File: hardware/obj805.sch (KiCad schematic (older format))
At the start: 37 parts, among them J0 Conn_with_rapi, U1 l293d

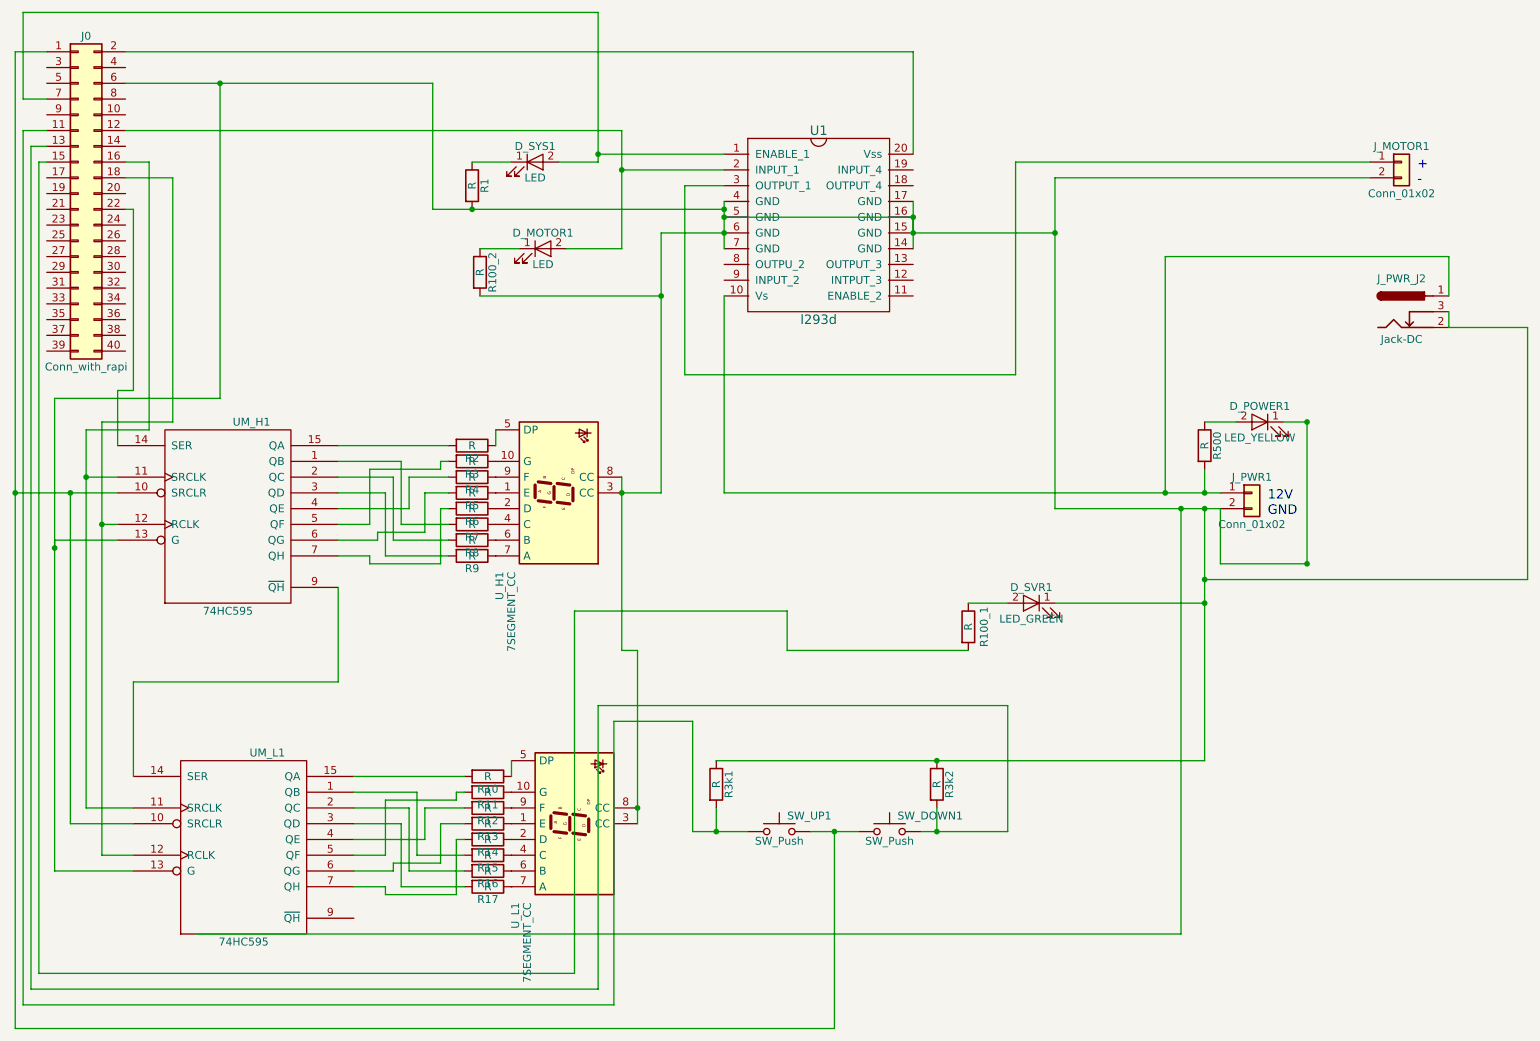
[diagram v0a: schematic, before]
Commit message: update
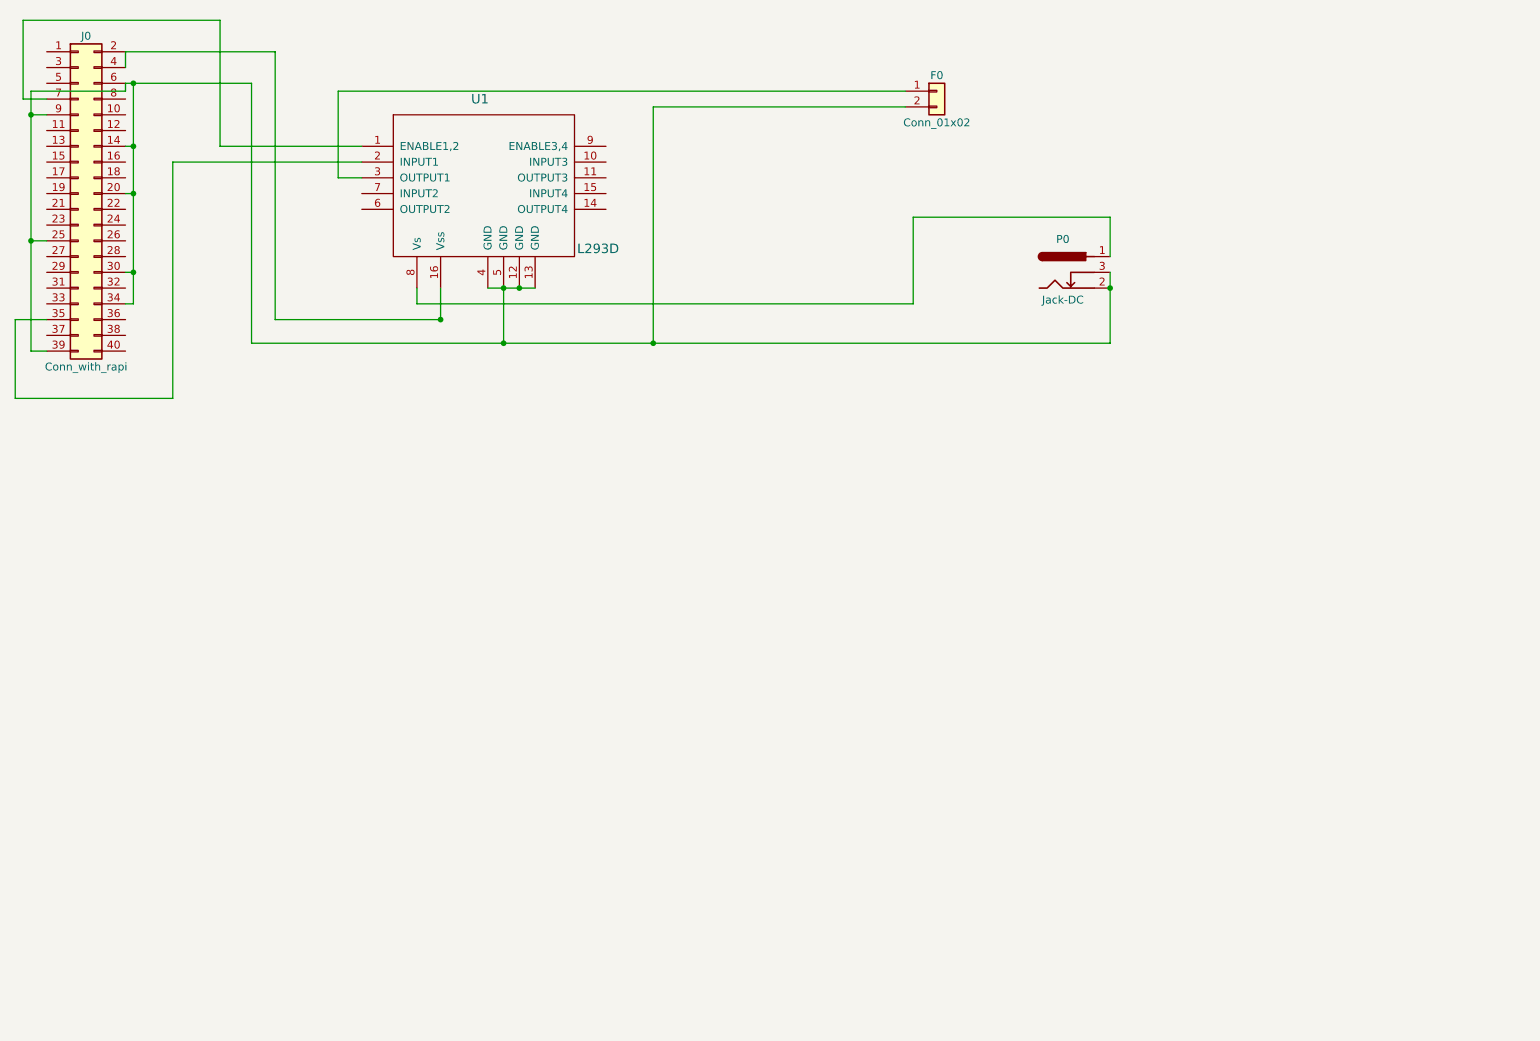
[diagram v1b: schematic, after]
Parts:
- removed D_MOTOR1, D_SYS1: LED, LEDs:LED_1206, symbol LED
- removed D_POWER1: LED_YELLOW, LEDs:LED_1206, symbol LED
- removed D_SVR1: LED_GREEN, LEDs:LED_1206, symbol LED
- removed J_MOTOR1, J_PWR1: Conn_01x02, Pin_Headers:Pin_Header_Straight_1x02_Pitch2.54mm, symbol Conn_01x02
- removed J_PWR_J2: Jack-DC, Connectors:JACK_ALIM, symbol Jack-DC
- removed R1, R10, R100_1, R100_2, R11, R12, R13, R14, R15, R16, R17, R2, R3, R3k1, R3k2, R4, R5, R500, R6, R7, R8, R9: R, Resistors_SMD:R_0805, symbol R
- removed SW_DOWN1, SW_UP1: SW_Push, Buttons_Switches_THT:SW_PUSH_6mm, symbol SW_Push
- removed U1: l293d, l293d:SOIC-20, symbol l293d
- removed UM_H1, UM_L1: 74HC595, SMD_Packages:SO-16-N, symbol 74HC595
- removed U_H1, U_L1: 7SEGMENT_CC, l293d:7SegmentLED_3611, symbol 7SEGMENT_CC
- added F0: Conn_01x02, Pin_Headers:Pin_Header_Straight_1x02_Pitch2.54mm, symbol Conn_01x02
- added P0: Jack-DC, Connectors:JACK_ALIM, symbol Jack-DC
- added U1: L293D, l293d:L293D, symbol L293D
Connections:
- net GND is gone; now on an unnamed net: J0.6 (Pin_6)
- net at J0.14 (Pin_14): now also J0.20 (Pin_20), J0.25 (Pin_25), J0.30 (Pin_30), J0.34 (Pin_34), J0.39 (Pin_39), J0.9 (Pin_9), F0.2 (Pin_2), P0.2, P0.3, U1.12 (GND), U1.13 (GND), U1.4 (GND), U1.5 (GND)
- net at J0.2 (Pin_2): now also J0.4 (Pin_4), U1.16 (Vss)
- net at J0.35 (Pin_35): now also U1.2 (INPUT1)
- net at J0.7 (Pin_7): now also U1.1 (ENABLE1,2)
- new net: P0.1, U1.8 (Vs)
- new net: F0.1 (Pin_1), U1.3 (OUTPUT1)
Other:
- note removed: "+\n-"
- note removed: "12V\nGND"
